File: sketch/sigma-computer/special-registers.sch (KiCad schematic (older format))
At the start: 12 parts

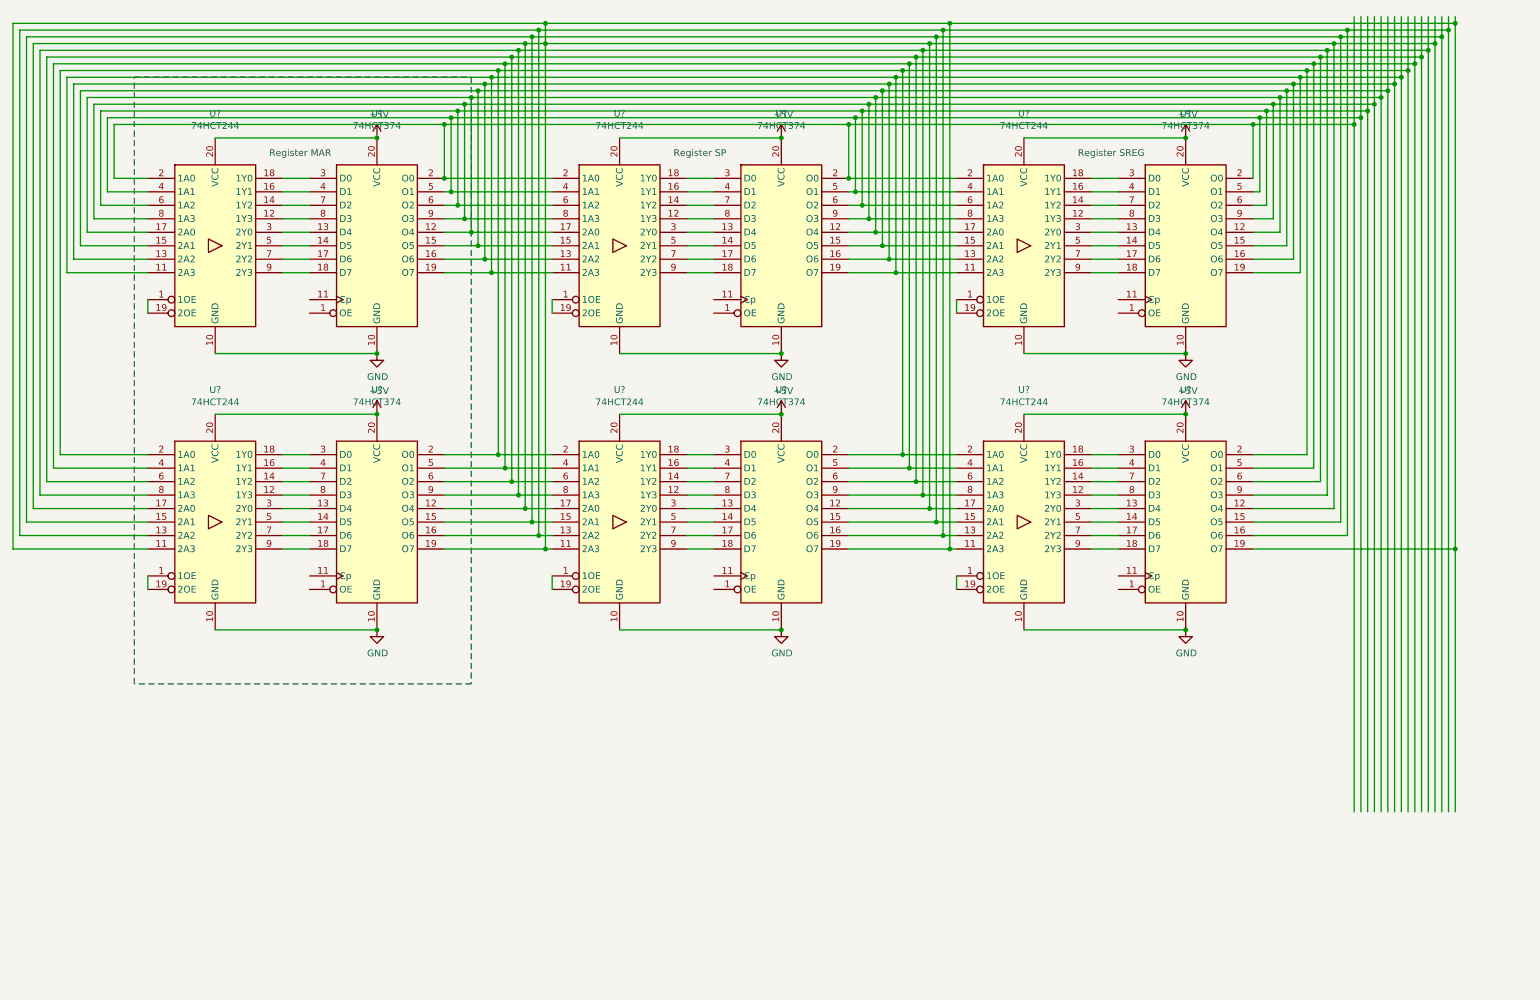
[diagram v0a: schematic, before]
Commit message: Changes in the schematic
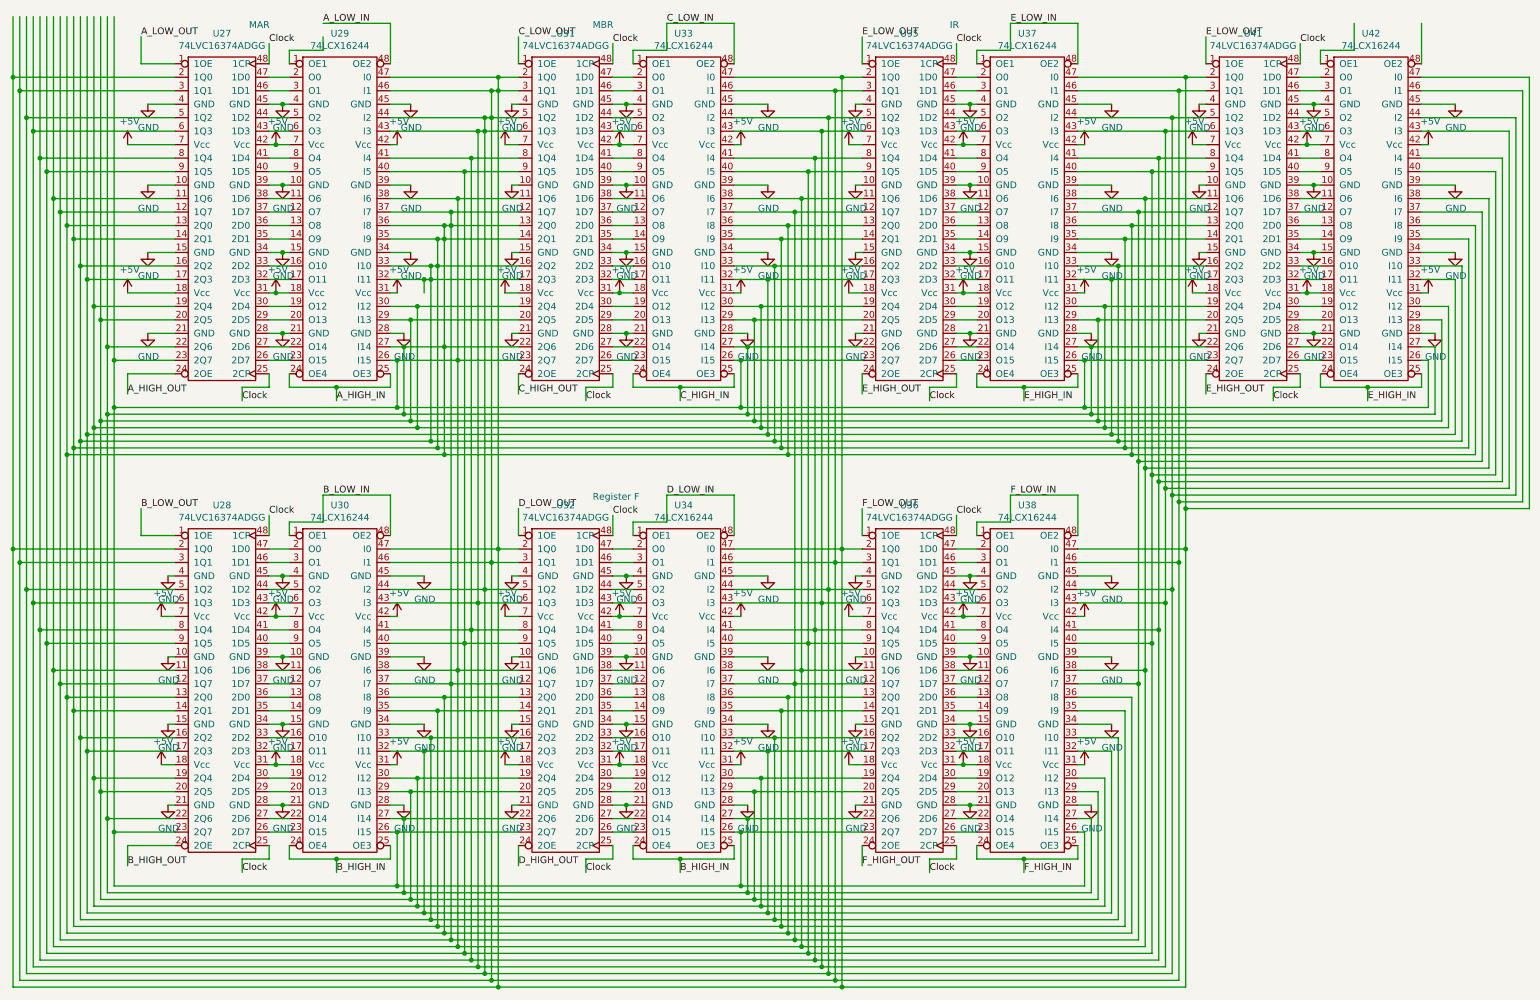
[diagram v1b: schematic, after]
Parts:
- removed U? (x6): 74HCT244, symbol 74xx:74HCT244
- removed U? (x6): 74HCT374, symbol 74xx:74HCT374
- added U27, U28, U31, U32, U35, U36, U41: 74LVC16374ADGG, symbol Additional74:74LVC16374ADGG
- added U29, U30, U33, U34, U37, U38, U42: 74LCX16244, symbol Additional74:74LCX16244
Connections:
- net labels added: A_HIGH_IN, A_HIGH_OUT, A_LOW_IN, A_LOW_OUT, B_HIGH_IN, B_HIGH_OUT, B_LOW_IN, B_LOW_OUT, C_HIGH_IN, C_HIGH_OUT, C_LOW_IN, C_LOW_OUT, Clock, D_HIGH_OUT, D_LOW_IN, D_LOW_OUT, E_HIGH_IN, E_HIGH_OUT, E_LOW_IN, E_LOW_OUT, F_HIGH_IN, F_HIGH_OUT, F_LOW_IN, F_LOW_OUT
- wire segments 320 -> 910
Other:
- note added: "IR"
- note added: "MAR\n"
- note added: "MBR"
- note added: "Register F\n"
- note removed: "Register MAR"
- note removed: "Register SP"
- note removed: "Register SREG"
